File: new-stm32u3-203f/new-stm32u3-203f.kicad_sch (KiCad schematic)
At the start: 31 parts, among them J1 Micro_SD_Card, J2 SJ-3524-SMT, J3 12401826E412A, SW1 SW_SPDT, U1 STM32U385RGT6Q, U2 TLV320DAC3203IRGER, X1 32.768kHz

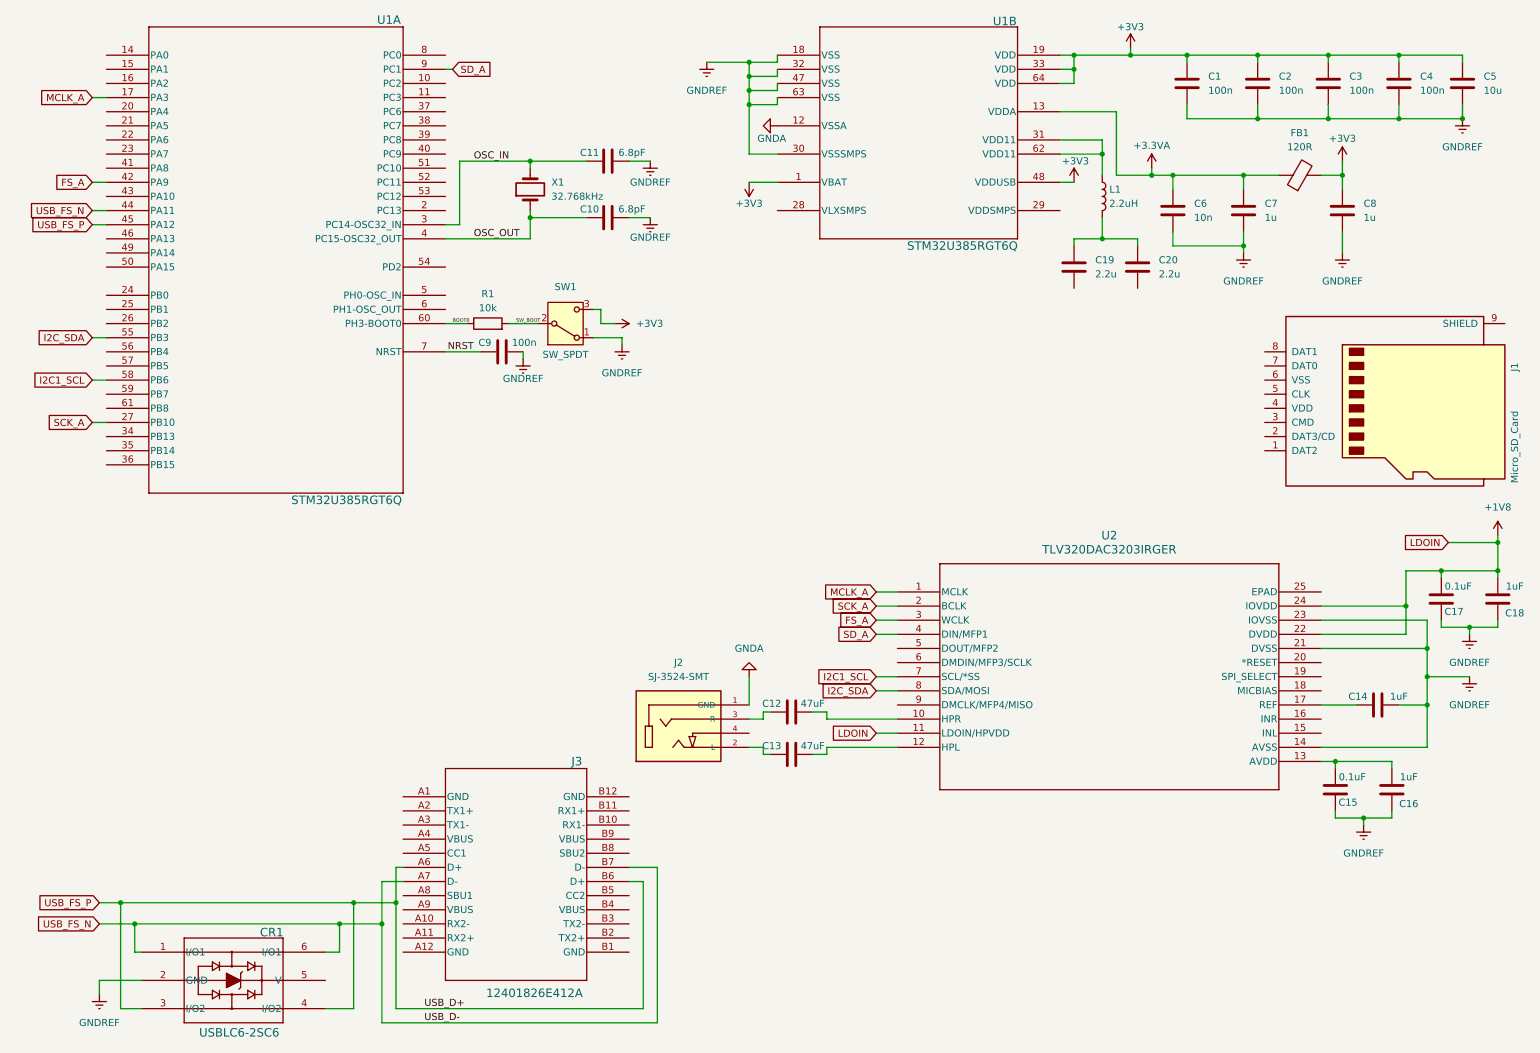
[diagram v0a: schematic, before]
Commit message: mcu power finished
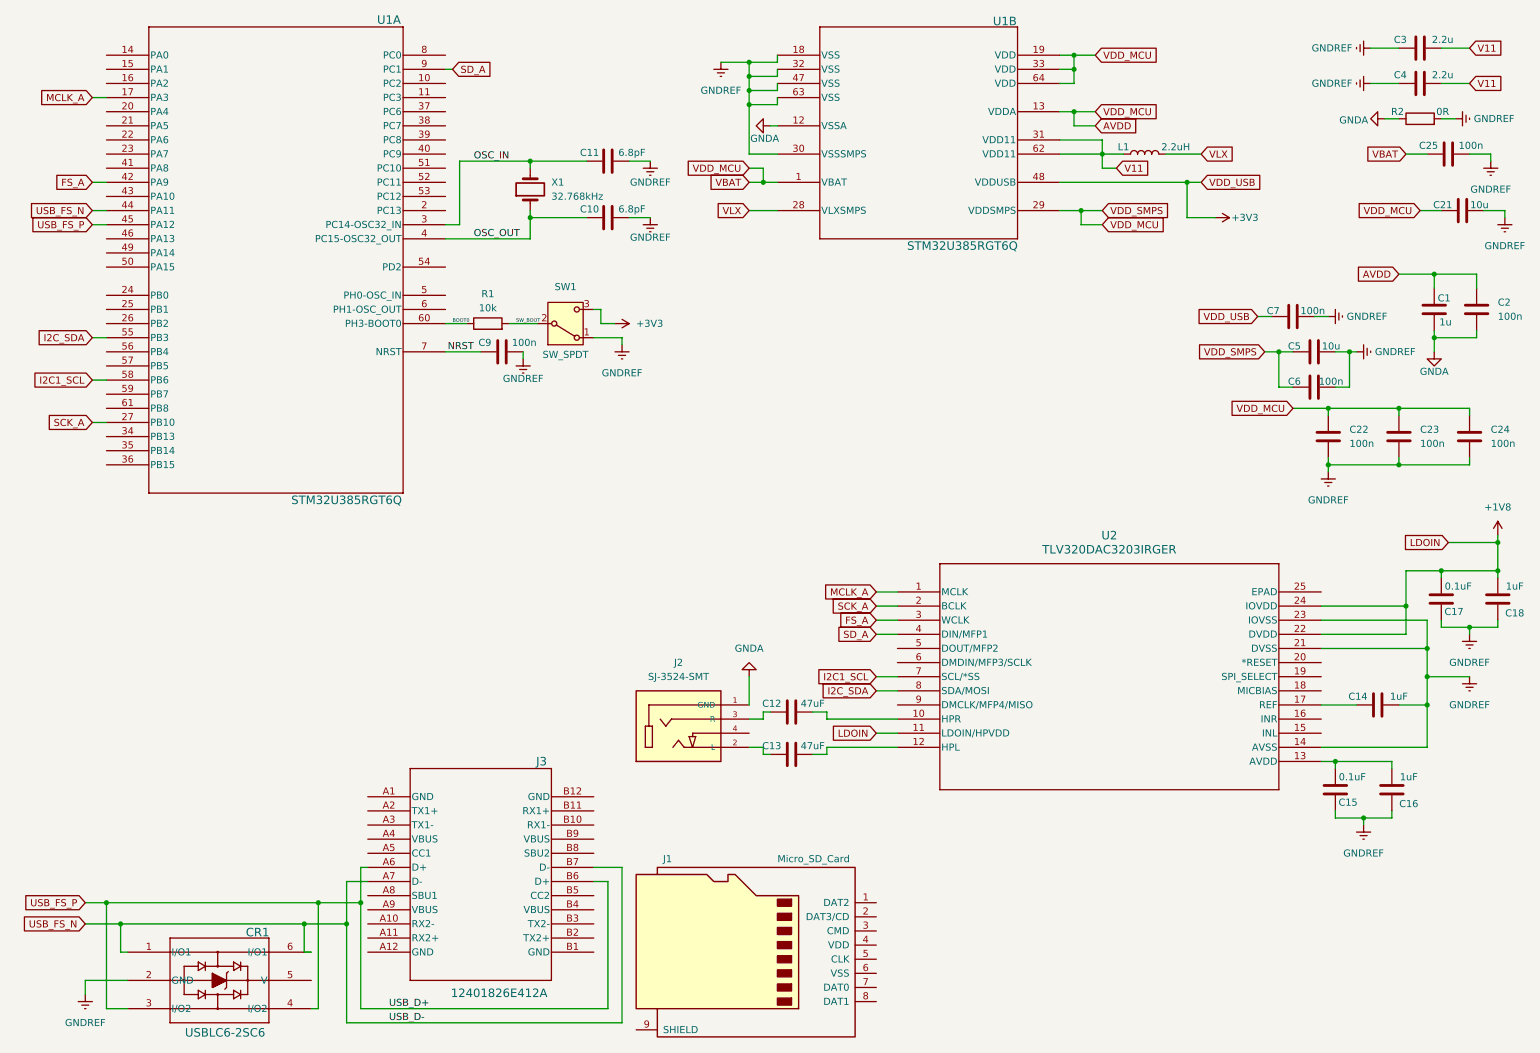
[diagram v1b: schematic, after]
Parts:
- removed C19, C20: 2.2u, symbol Device:C
- removed C8: 1u, symbol Device:C
- removed FB1: 120R, symbol Device:FerriteBead
- added C21: 10u, symbol Device:C
- added C22, C23, C24, C25: 100n, symbol Device:C
- added R2: 0R, symbol Device:R
- C1: value 100n -> 1u
- C3, C4: value 100n -> 2.2u
- C6: value 10n -> 100n
- C7: value 1u -> 100n
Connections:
- net +3V3: now also C7.2; no longer C1.1, C2.1, C3.1, C4.1, C5.1, U1.1 (VBAT), U1.19 (VDD), U1.33 (VDD), U1.64 (VDD)
- net GNDA: now also C1.1, C2.1, R2.1
- net GNDREF: now also C5.1, C6.1, C7.1, C21.1, C22.1, C23.1, C24.1, C25.1, R2.2; no longer C1.2, C2.2, C5.2, C6.2, C7.2
- net VLX: now reaches L1.2
- net VLX: now also U1.28 (VLXSMPS)
- net V11: now reaches L1.1, U1.31 (VDD11), U1.62 (VDD11)
- net V11: now also C3.1, C4.1
- net AVDD: now reaches U1.29 (VDDSMPS)
- net AVDD: now also C1.2, C2.2, C5.2, C6.2, U1.1 (VBAT), U1.13 (VDDA), U1.19 (VDD), U1.33 (VDD), U1.64 (VDD), C21.2, C22.2, C23.2, C24.2, C25.2
- removed net +3.3VA: C6.1, C7.1, U1.13 (VDDA)
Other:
- moved on the sheet: CR1, J1, J3, L1
